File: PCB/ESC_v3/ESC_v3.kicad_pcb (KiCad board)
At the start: 4 copper layers, 42 x 83.5 mm, 145 parts, among them IC1 TLV77333PDBVR, IC2 TCAN3414DR, IC3 DRV8323SRTAR, J1 Conn_01x04_Pin, J10 Conn_01x01_Pin, J3 Conn_01x01_Pin, J4 Conn_01x01_Pin, J5 Conn_01x01_Pin, J6 Conn_01x01_Pin, J7 Conn_01x01_Pin, J8 Conn_01x01_Pin, J9 Conn_01x01_Pin, Q1 NTMFS5C670NLT1G, Q2 NTMFS5C670NLT1G, Q3 NTMFS5C670NLT1G, Q4 NTMFS5C670NLT1G, Q5 NTMFS5C670NLT1G, Q6 NTMFS5C670NLT1G, U3 STM32G474CETx, Y2 24MHz

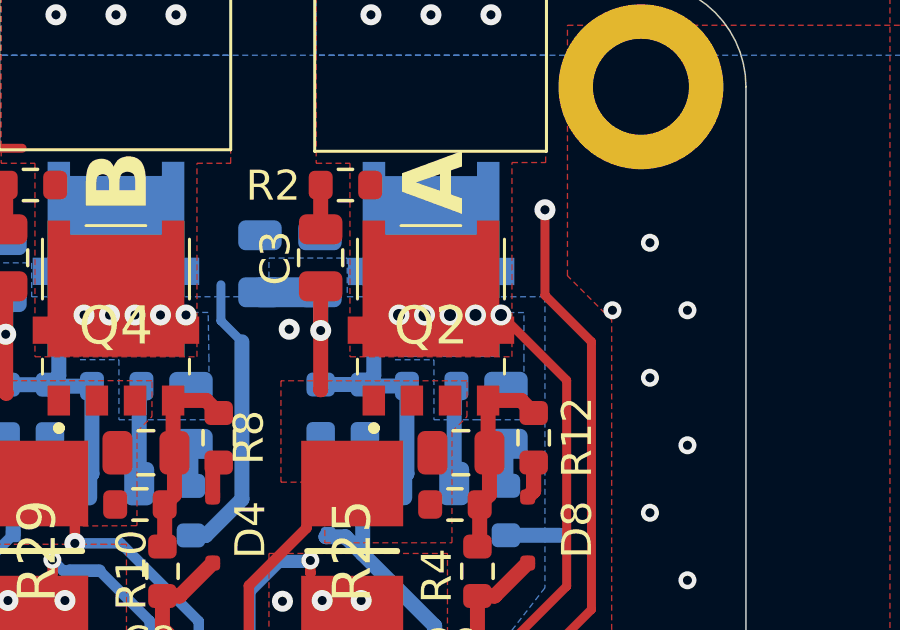
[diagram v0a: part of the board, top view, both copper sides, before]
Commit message: Layout update
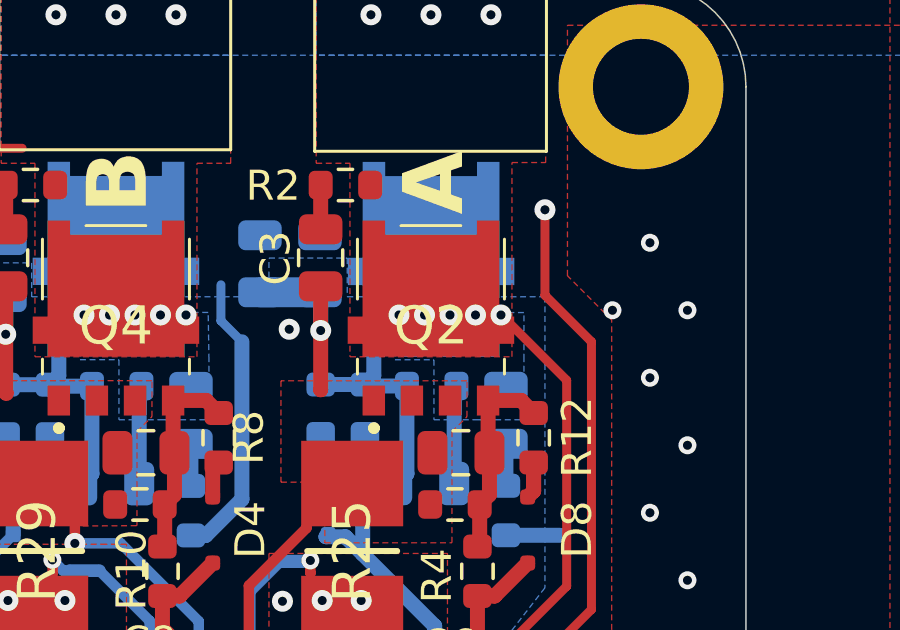
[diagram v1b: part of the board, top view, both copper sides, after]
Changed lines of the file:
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@@
 		(at 157.185 45.00775)
 		(size 0.7)
-		(drill 0.4)
+		(drill 0.3)
 		(layers "F.Cu" "B.Cu")
 		(tenting front back)
@@
 		(at 156.335 45.00775)
 		(size 0.7)
-		(drill 0.4)
+		(drill 0.3)
 		(layers "F.Cu" "B.Cu")
 		(tenting front back)
@@
 		(at 154.635 45.00775)
 		(size 0.7)
-		(drill 0.4)
+		(drill 0.3)
 		(layers "F.Cu" "B.Cu")
 		(tenting front back)
@@
 		(at 158.035 45.00775)
 		(size 0.7)
-		(drill 0.4)
+		(drill 0.3)
 		(layers "F.Cu" "B.Cu")
 		(tenting front back)
@@
 		(at 155.485 45.00775)
 		(size 0.7)
-		(drill 0.4)
+		(drill 0.3)
 		(layers "F.Cu" "B.Cu")
 		(tenting front back)
@@
 	)
 	(zone
-		(net 3)
-		(net_name "V_A_PHASE")
-		(layer "F.Cu")
-		(name "$teardrop_padvia$")
-		(hatch none 0.1)
-		(priority 30277)
-		(attr
-			(teardrop
-				(type padvia)
-			)
-		)
-		(connect_pads yes
-			(clearance 0)
-		)
-		(min_thickness 0.0254)
-		(filled_areas_thickness no)
-		(fill yes
-			(thermal_gap 0.5)
-			(thermal_bridge_width 0.5)
-			(island_removal_mode 1)
-			(island_area_min 10)
-		)
-		(polygon
-			(pts
-				(xy 158.152196 44.900064) (xy 158.067367 44.841369) (xy 157.964964 44.815382) (xy 157.85635 44.826315)
-				(xy 157.806513 44.845827) (xy 157.762811 44.874004) (xy 157.729253 44.907722) (xy 157.704456 44.948089)
-				(xy 157.69087 44.990298) (xy 157.687168 45.037314) (xy 157.691725 45.076032) (xy 158.034293 45.007043)
-				(xy 157.691725 45.076032) (xy 157.702226 45.104546) (xy 157.718419 45.118527) (xy 157.759323 45.11773)
-				(xy 157.79492 45.105856) (xy 157.868926 45.086297) (xy 157.905715 45.090474) (xy 157.940064 45.112196)
-			)
-		)
-	)
-	(zone
 		(net 26)
 		(net_name "Net-(D8-A)")
@@
 			)
 		)
+	)
+	(zone
+		(net 3)
+		(net_name "V_A_PHASE")
+		(layer "F.Cu")
+		(name "$teardrop_padvia$")
+		(hatch none 0.1)
+		(priority 30000)
+		(attr
+			(teardrop
+				(type padvia)
+			)
+		)
+		(connect_pads yes
+			(clearance 0)
+		)
+		(min_thickness 0.0254)
+		(filled_areas_thickness no)
+		(fill yes
+			(thermal_gap 0.5)
+			(thermal_bridge_width 0.5)
+			(island_removal_mode 1)
+			(island_area_min 10)
+		)
+		(polygon
+			(pts
+				(xy 158.152196 44.900064) (xy 158.067367 44.841369) (xy 157.964964 44.815382) (xy 157.85635 44.826315)
+				(xy 157.806513 44.845827) (xy 157.762811 44.874004) (xy 157.729253 44.907722) (xy 157.704456 44.948089)
+				(xy 157.69087 44.990298) (xy 157.687168 45.037314) (xy 157.691725 45.076032) (xy 158.034293 45.007043)
+				(xy 157.691725 45.076032) (xy 157.702226 45.104546) (xy 157.718419 45.118527) (xy 157.759323 45.11773)
+				(xy 157.79492 45.105856) (xy 157.868926 45.086297) (xy 157.905715 45.090474) (xy 157.940064 45.112196)
+			)
+		)

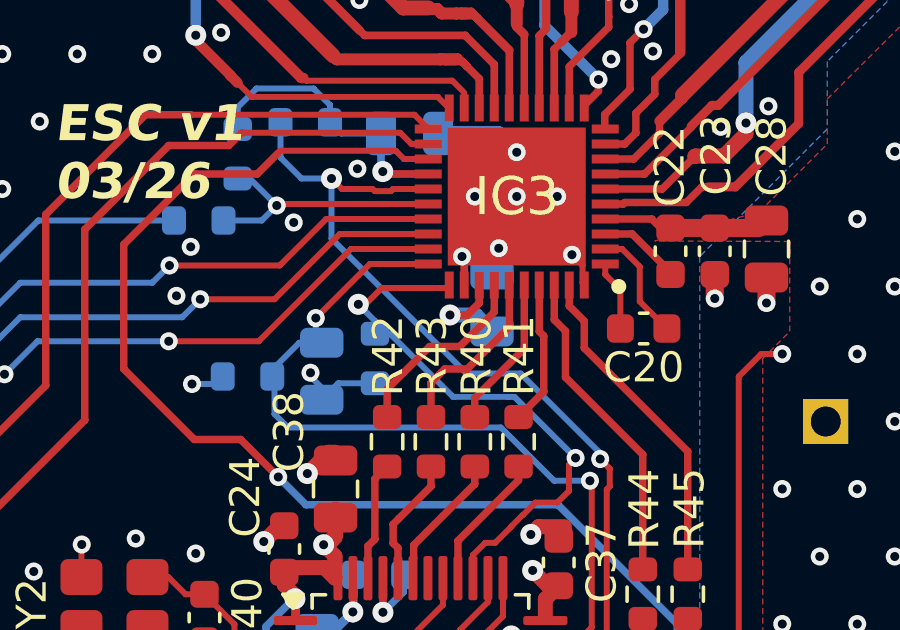
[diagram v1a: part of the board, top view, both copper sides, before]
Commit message: Update
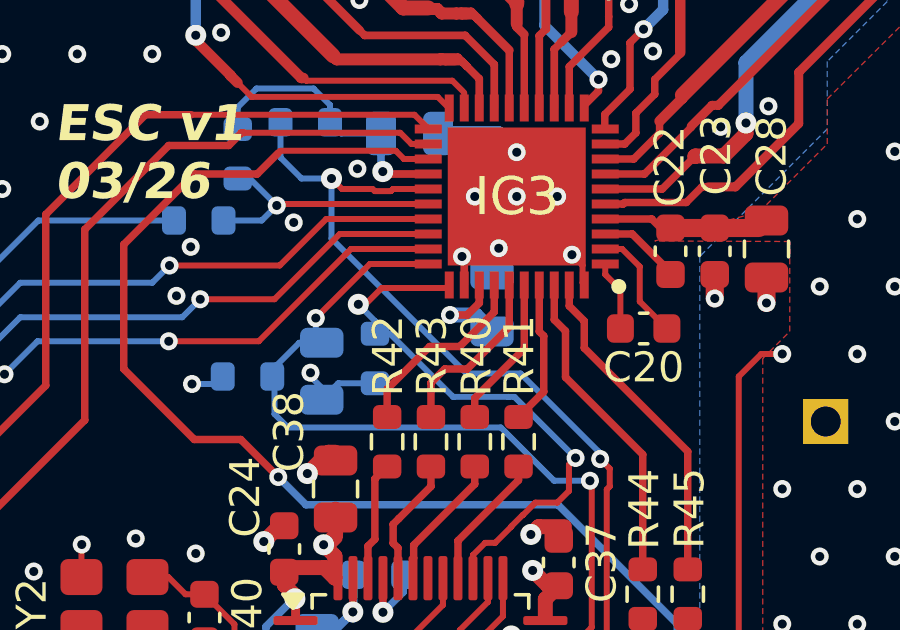
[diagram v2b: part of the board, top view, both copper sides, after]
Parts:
- C32: value 100n -> 10n
- C46, C47, C48: value 100p -> 1000p
- R10, R17, R20, R4, R5, R9: value 4.7Ω -> 10R
- R46, R47, R48: value 33 -> 1k
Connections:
- net TIM17_CH1 renamed TIM8_CH3
- net TIM17_CH1N renamed TIM3_CH4
- net V_BAT renamed +VBAT
- C21 pad 1: +3V3 -> Net-(IC3-DVDD)
- IC3 pad 33: +3V3 -> Net-(IC3-DVDD)
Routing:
- net +3V3: track 113.4 -> 106.8 mm, vias 11 -> 10
- net Net-(IC3-DVDD): track 0.00 -> 3.38 mm, vias 0 -> 1
